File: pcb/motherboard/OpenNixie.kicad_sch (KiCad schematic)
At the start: 43 parts, among them J1 Conn_01x02, J10 Nixie_Conn_12P, J2 Conn_01x03, J3 Nixie_Conn_4P, J4 Conn_01x04, J5 Conn_01x03, J6 12V, J7 Nixie_Conn_12P, J8 Nixie_Conn_12P, J9 Nixie_Conn_12P, Q1 MPSA42, Q2 S8050, Q3 TK8P65W, U1 LM7805_TO220, U2 NE555P, U3 NE555P, U4 MAX1771CSA, U5 74LS138, U6 74HC595, U7 74LS138

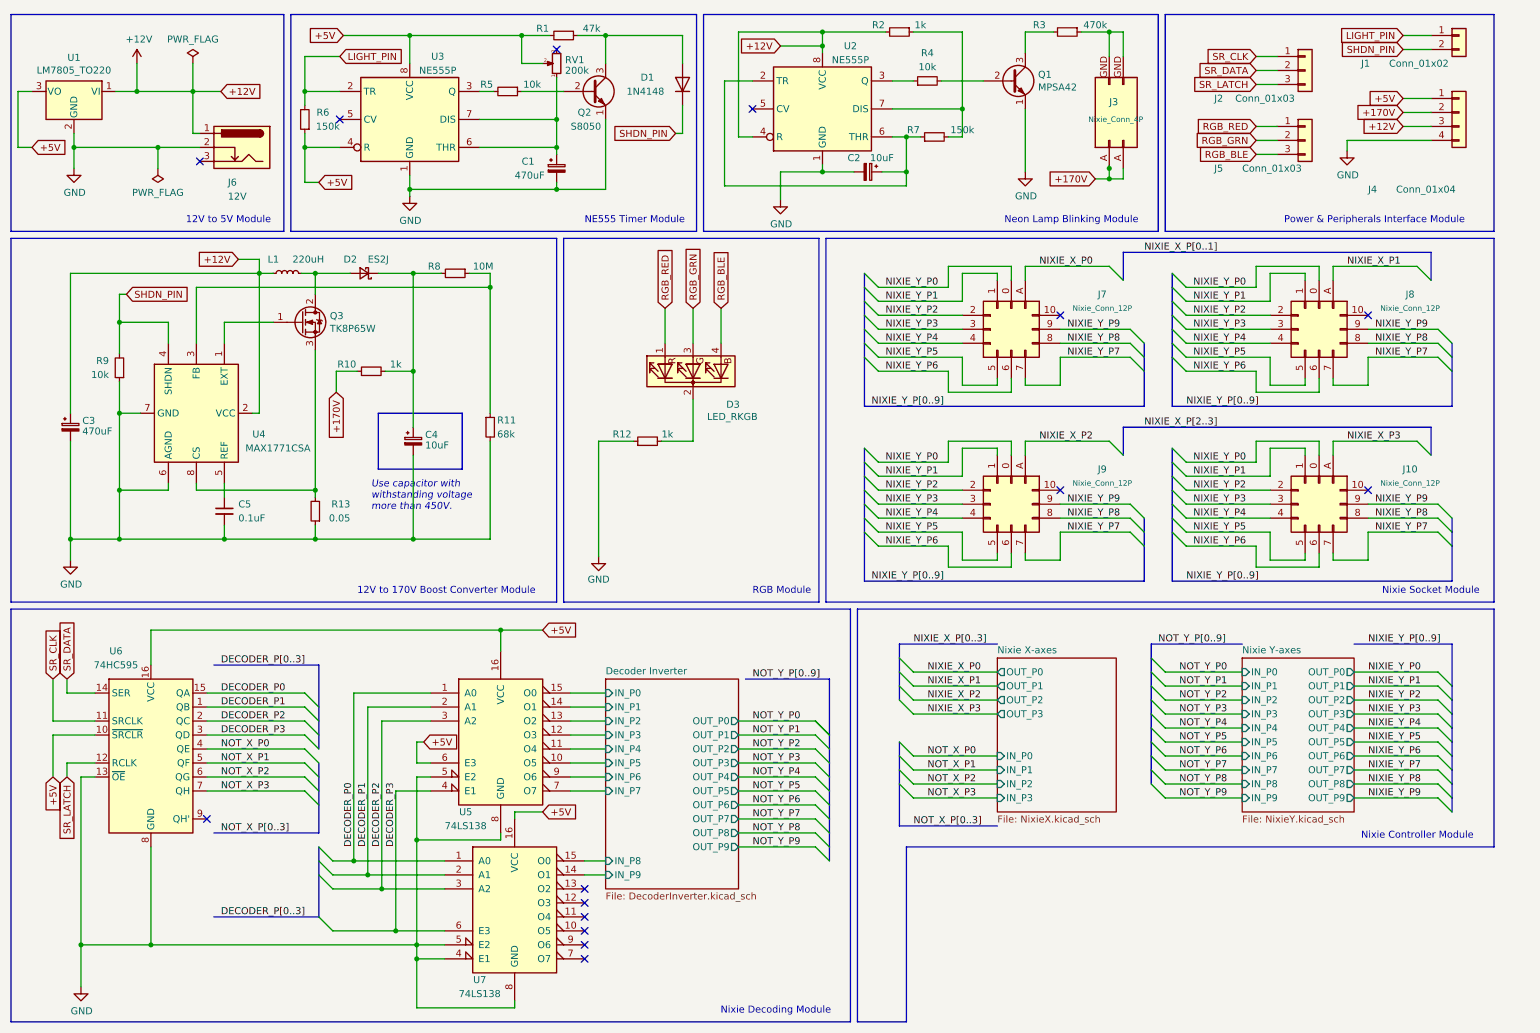
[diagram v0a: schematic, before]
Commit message: PCB updated
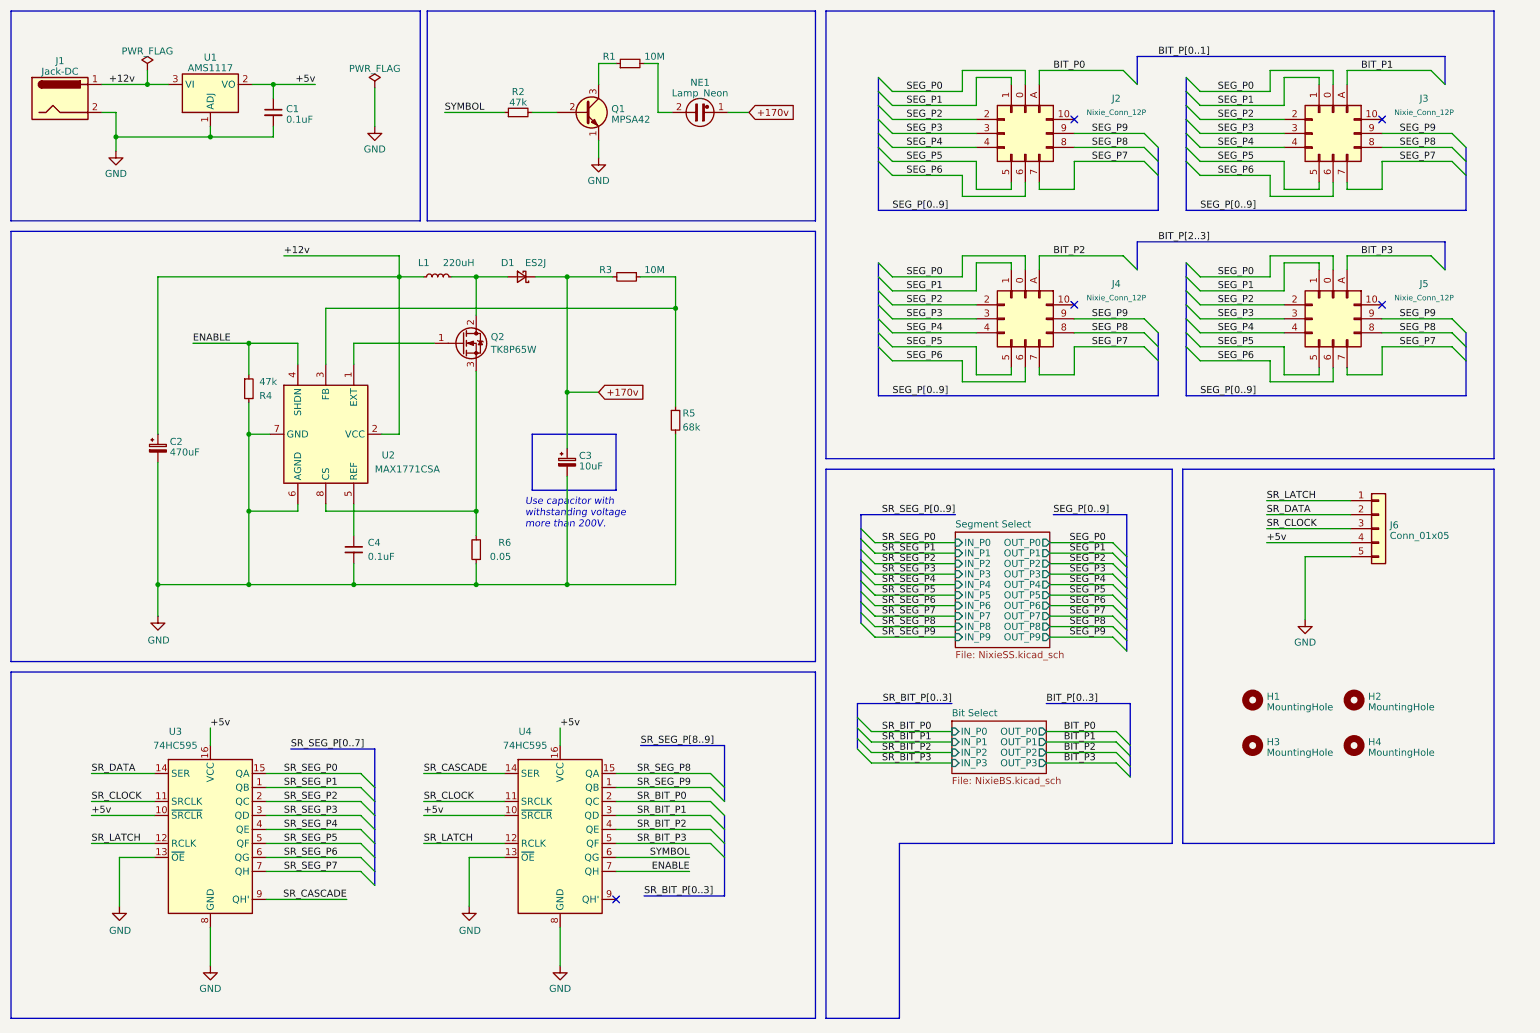
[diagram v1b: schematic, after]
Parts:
- removed C1: 470uF, Capacitor_THT:CP_Radial_D8.0mm_P3.50mm, symbol Device:C_Polarized_Small
- removed C2: 10uF, Capacitor_THT:CP_Radial_D5.0mm_P2.00mm, symbol Device:C_Polarized_Small
- removed D1: 1N4148, Diode_THT:D_DO-35_SOD27_P2.54mm_Vertical_AnodeUp, symbol Diode:1N4148
- removed D3: LED_RKGB, LED_THT:LED_D5.0mm-4_RGB_Wide_Pins, symbol Device:LED_RKGB
- removed J1: Conn_01x02, Connector_JST:JST_EH_B2B-EH-A_1x02_P2.50mm_Vertical, symbol Connector_Generic:Conn_01x02
- removed J2, J5: Conn_01x03, Connector_JST:JST_EH_B3B-EH-A_1x03_P2.50mm_Vertical, symbol Connector_Generic:Conn_01x03
- removed J3: Nixie_Conn_4P, Nixie_Clock:Nixie_Conn_4P, symbol Nixie_Clock:Nixie_Conn_4P
- removed J4: Conn_01x04, Connector_JST:JST_EH_B4B-EH-A_1x04_P2.50mm_Vertical, symbol Connector_Generic:Conn_01x04
- removed J6: 12V, Connector_BarrelJack:BarrelJack_Horizontal, symbol Connector:Barrel_Jack_Switch_Pin3Ring
- removed Q1: MPSA42, Package_TO_SOT_THT:TO-92_Inline, symbol Transistor_BJT:MPSA42
- removed Q2: S8050, Package_TO_SOT_THT:TO-92_Inline, symbol Transistor_BJT:S8050
- removed R10: 1k, Resistor_THT:R_Axial_DIN0309_L9.0mm_D3.2mm_P12.70mm_Horizontal, symbol Device:R_Small
- removed R12: 1k, Resistor_THT:R_Axial_DIN0204_L3.6mm_D1.6mm_P5.08mm_Horizontal, symbol Device:R_Small
- removed R3: 470k, Resistor_THT:R_Axial_DIN0204_L3.6mm_D1.6mm_P5.08mm_Horizontal, symbol Device:R_Small
- removed R4, R5: 10k, Resistor_THT:R_Axial_DIN0204_L3.6mm_D1.6mm_P5.08mm_Horizontal, symbol Device:R_Small
- removed R6, R7: 150k, Resistor_THT:R_Axial_DIN0204_L3.6mm_D1.6mm_P5.08mm_Horizontal, symbol Device:R_Small
- removed RV1: 200k, Potentiometer_THT:Potentiometer_Vishay_T73YP_Vertical, symbol Device:R_Potentiometer_Small
- removed U1: LM7805_TO220, Package_TO_SOT_THT:TO-220-3_Vertical, symbol Regulator_Linear:LM7805_TO220
- removed U2, U3: NE555P, Package_DIP:DIP-8_W7.62mm, symbol Timer:NE555P
- removed U5, U7: 74LS138, Package_DIP:DIP-16_W7.62mm, symbol 74xx:74LS138
- added C1: 0.1uF, Capacitor_THT:C_Disc_D3.0mm_W2.0mm_P2.50mm, symbol Device:C_Small
- added H1, H2, H3, H4: MountingHole, MountingHole:MountingHole_3.2mm_M3, symbol Mechanical:MountingHole
- added J1: Jack-DC, Connector_BarrelJack:BarrelJack_Horizontal, symbol Connector:Jack-DC
- added J6: Conn_01x05, Connector_PinHeader_2.54mm:PinHeader_1x05_P2.54mm_Vertical, symbol Connector_Generic:Conn_01x05
- added NE1: Lamp_Neon, Connector_PinSocket_2.54mm:PinSocket_1x02_P2.54mm_Vertical, symbol Device:Lamp_Neon
- added Q1: MPSA42, Package_TO_SOT_THT:TO-92_Inline, symbol PCM_Transistor_BJT_AKL:MPSA42
- added U1: AMS1117, Package_TO_SOT_SMD:SOT-223-3_TabPin2, symbol Regulator_Linear:AMS1117
- added U4: 74HC595, Package_DIP:DIP-16_W7.62mm, symbol 74xx:74HC595
- R1: value 47k -> 10M
- R2: value 1k -> 47k
- R4: renamed from R9; value 10k -> 47k
- renumbered C3 to C2, C4 to C3, C5 to C4, D2 to D1, J7 to J2, J8 to J3, J9 to J4, J10 to J5, Q3 to Q2, R8 to R3, R11 to R5, R13 to R6, U4 to U2, U6 to U3
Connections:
- net GND: now also R4.2, C1.2, J1.2, J6.5 (Pin_5), Q1.1 (E), U1.1 (ADJ), U4.13 (~{OE}), U4.8 (GND); no longer R4.1
- net SR_DATA: now also J6.2 (Pin_2)
- net SR_LATCH: now also J6.1 (Pin_1), U4.12 (RCLK)
- net +170v: now reaches C3.1, D1.1 (K), R3.2
- net +170v: now also NE1.1
- net at R1.1: now also Q1.3 (C)
- net SR_CASCADE: now reaches U3.9 (QH')
- net SR_CASCADE: now also U4.14 (SER)
- net SYMBOL: now reaches R2.1
- net SYMBOL: now also U4.6 (QG)
- net +12V renamed +12v
- net +12v: now also J1.1, U1.3 (VI); no longer R2.2
- net +5V renamed +5v
- net +5v: now also C1.1, J6.4 (Pin_4), U1.2 (VO), U4.10 (~{SRCLR}), U4.16 (VCC); no longer R1.2
- net DECODER_P0 renamed SR_SEG_P0
- net DECODER_P1 renamed SR_SEG_P1
- net DECODER_P2 renamed SR_SEG_P2
- net DECODER_P3 renamed SR_SEG_P3
- net NIXIE_X_P0 renamed BIT_P0
- net NIXIE_X_P1 renamed BIT_P1
- net NIXIE_X_P2 renamed BIT_P2
- net NIXIE_X_P3 renamed BIT_P3
- net NIXIE_Y_P0 renamed SEG_P0
- net NIXIE_Y_P1 renamed SEG_P1
- net NIXIE_Y_P2 renamed SEG_P2
- net NIXIE_Y_P3 renamed SEG_P3
- net NIXIE_Y_P4 renamed SEG_P4
- net NIXIE_Y_P5 renamed SEG_P5
- net NIXIE_Y_P6 renamed SEG_P6
- net NIXIE_Y_P7 renamed SEG_P7
- net NIXIE_Y_P8 renamed SEG_P8
- net NIXIE_Y_P9 renamed SEG_P9
- net NOT_X_P0 renamed SR_SEG_P4
- net NOT_X_P1 renamed SR_SEG_P5
- net NOT_X_P2 renamed SR_SEG_P6
- net NOT_X_P3 renamed SR_SEG_P7
- net SHDN_PIN renamed ENABLE
- net ENABLE: now also R4.1, U4.7 (QH); no longer R4.2
- net SR_CLK renamed SR_CLOCK
- net SR_CLOCK: now also J6.3 (Pin_3), U4.11 (SRCLK)
- new net: Q1.2 (B), R2.2
- new net: NE1.2, R1.2
- new net SR_BIT_P0: U4.2 (QC)
- new net SR_BIT_P1: U4.3 (QD)
- new net SR_BIT_P2: U4.4 (QE)
- new net SR_BIT_P3: U4.5 (QF)
- new net SR_SEG_P8: U4.15 (QA)
- new net SR_SEG_P9: U4.1 (QB)
- no-connect marks 15 -> 5
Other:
- removed sheet Decoder Inverter
- removed sheet Nixie X-axes
- removed sheet Nixie Y-axes
- added sheet Bit Select (NixieBS.kicad_sch)
- added sheet Segment Select (NixieSS.kicad_sch)
- note added: "Use capacitor with withstanding voltage more than 200V."
- note removed: "12V to 170V Boost Converter Module"
- note removed: "12V to 5V Module"
- note removed: "NE555 Timer Module"
- note removed: "Neon Lamp Blinking Module"
- note removed: "Nixie Controller Module"
- note removed: "Nixie Decoding Module"
- note removed: "Nixie Socket Module"
- note removed: "Power & Peripherals Interface Module"
- note removed: "RGB Module"
- note removed: "Use capacitor with withstanding voltage more than 450V."
- moved on the sheet: C2, C3, C4, D1, J2, J3, J4, J5, L1, Q2, R3, R4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
